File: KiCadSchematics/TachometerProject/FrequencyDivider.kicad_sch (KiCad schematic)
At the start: 7 parts, among them U1 74LS90, U2 74LS90

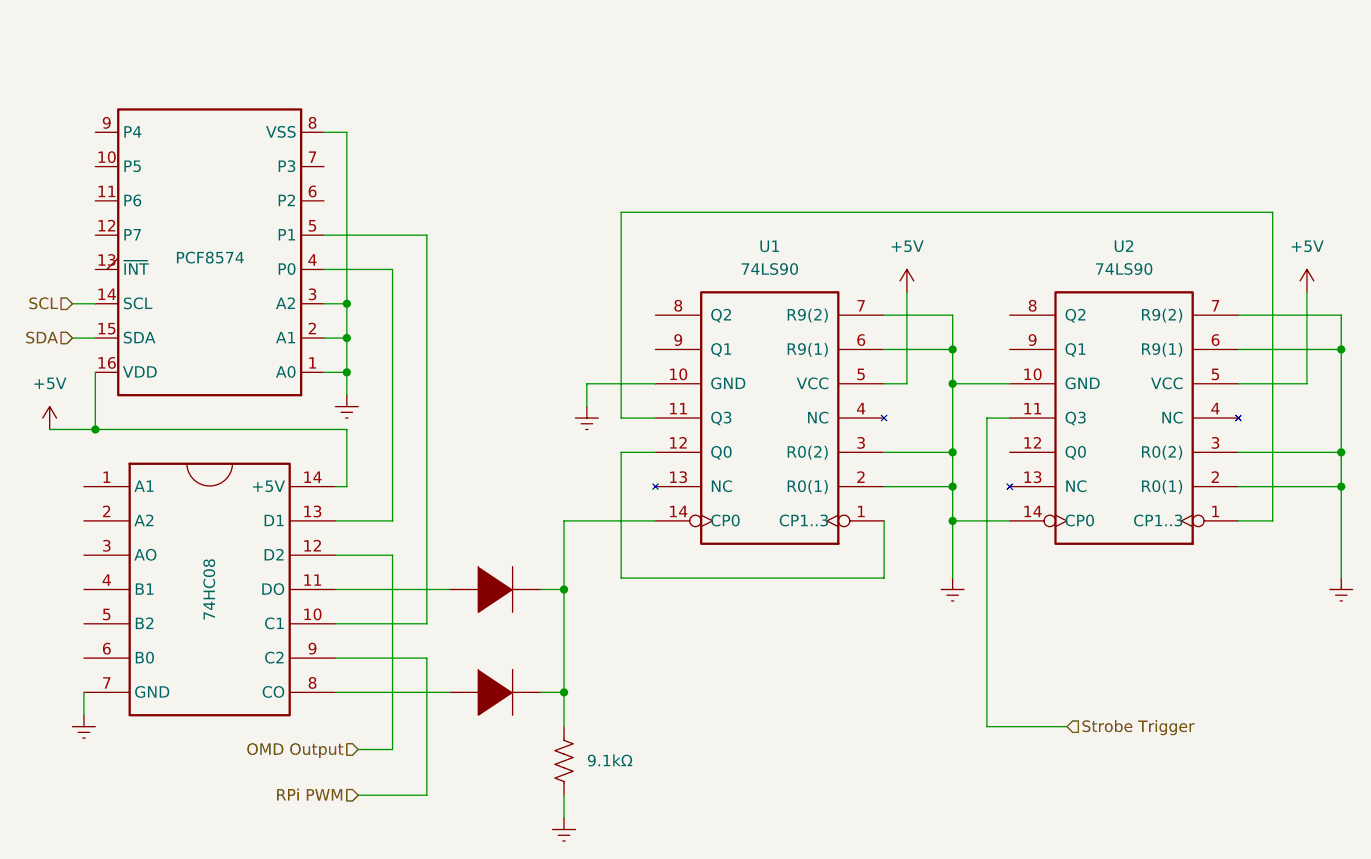
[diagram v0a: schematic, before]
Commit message: Updated circuit diagrams
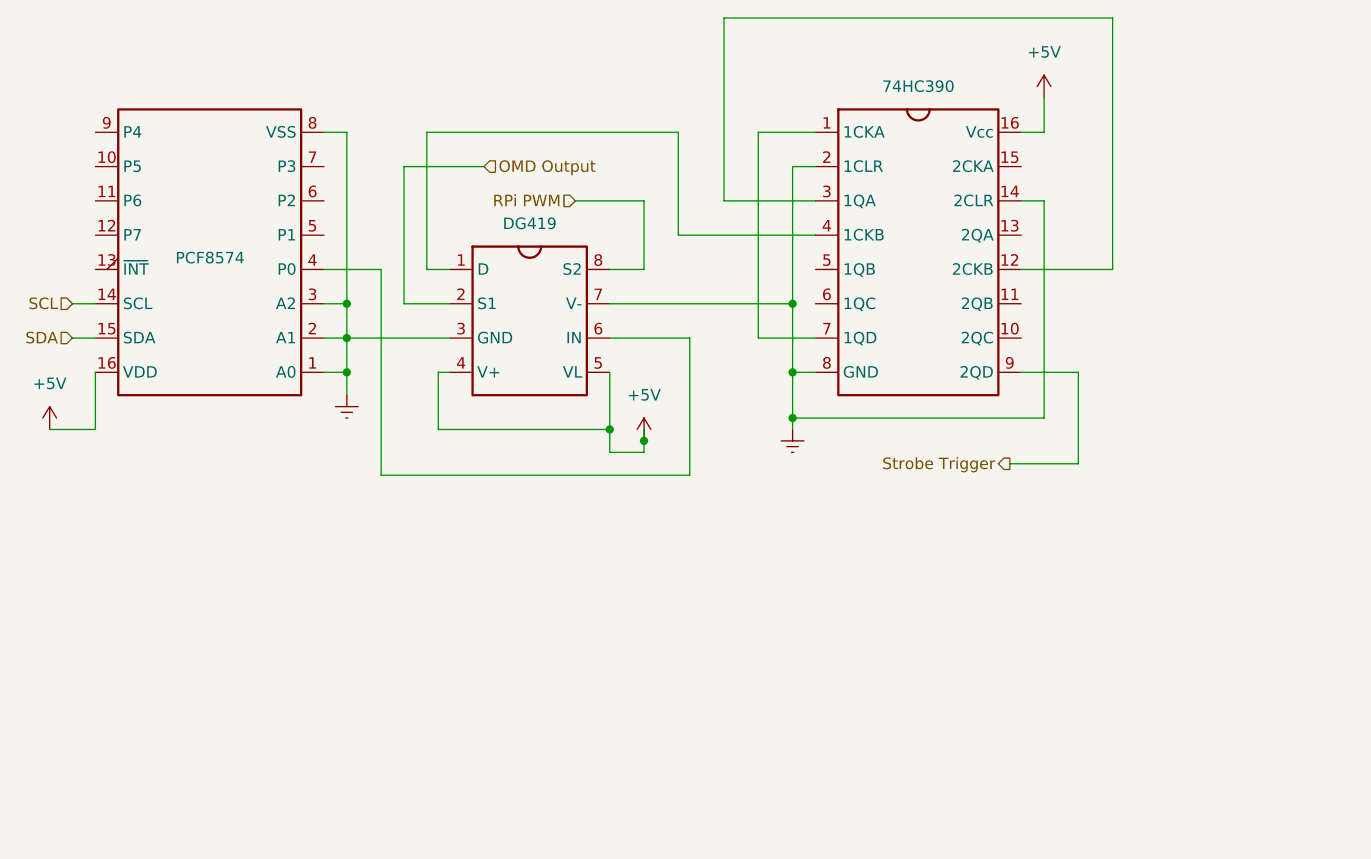
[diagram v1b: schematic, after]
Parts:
- removed D? (x2): DIODE, symbol pspice:DIODE
- removed R?: 9.1kΩ, symbol Device:R_US
- removed U1, U2: 74LS90, symbol 74xx:74LS90
- removed U?: 74HC08, symbol EGR_270:74HC08
- added U?: DG419, symbol EGR_270:DG419
- added U?: 74HC390, symbol EGR_270:74HC390
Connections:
- net +5V: now also U?.16 (Vcc), U?.4 (V+), U?.5 (VL)
- net Earth: now also U?.14 (2CLR), U?.2 (1CLR), U?.3 (GND), U?.7 (V-), U?.8 (GND)
- net OMD Output: now also U?.2 (S1)
- net RPi PWM: now also U?.8 (S2)
- net Strobe Trigger: now also U?.9 (2QD)
- net at U?.4 (P0): now also U?.6 (IN)
- new net: U?.1 (D), U?.4 (1CKB)
- new net: U?.1 (1CKA), U?.7 (1QD)
- new net: U?.12 (2CKB), U?.3 (1QA)
